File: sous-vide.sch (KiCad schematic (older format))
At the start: 25 parts, among them J2 Conn_01x02, J3 Conn_01x02, J5 Conn_01x02, Q1 2N3904, SW1 SW_Push_Dual, SW2 SW_Push_Dual, U1 node_mcu1.0, U2 RAC01, U3 G5LE, U4 LCD_Backpack, U5 P090S-04F20BR10K

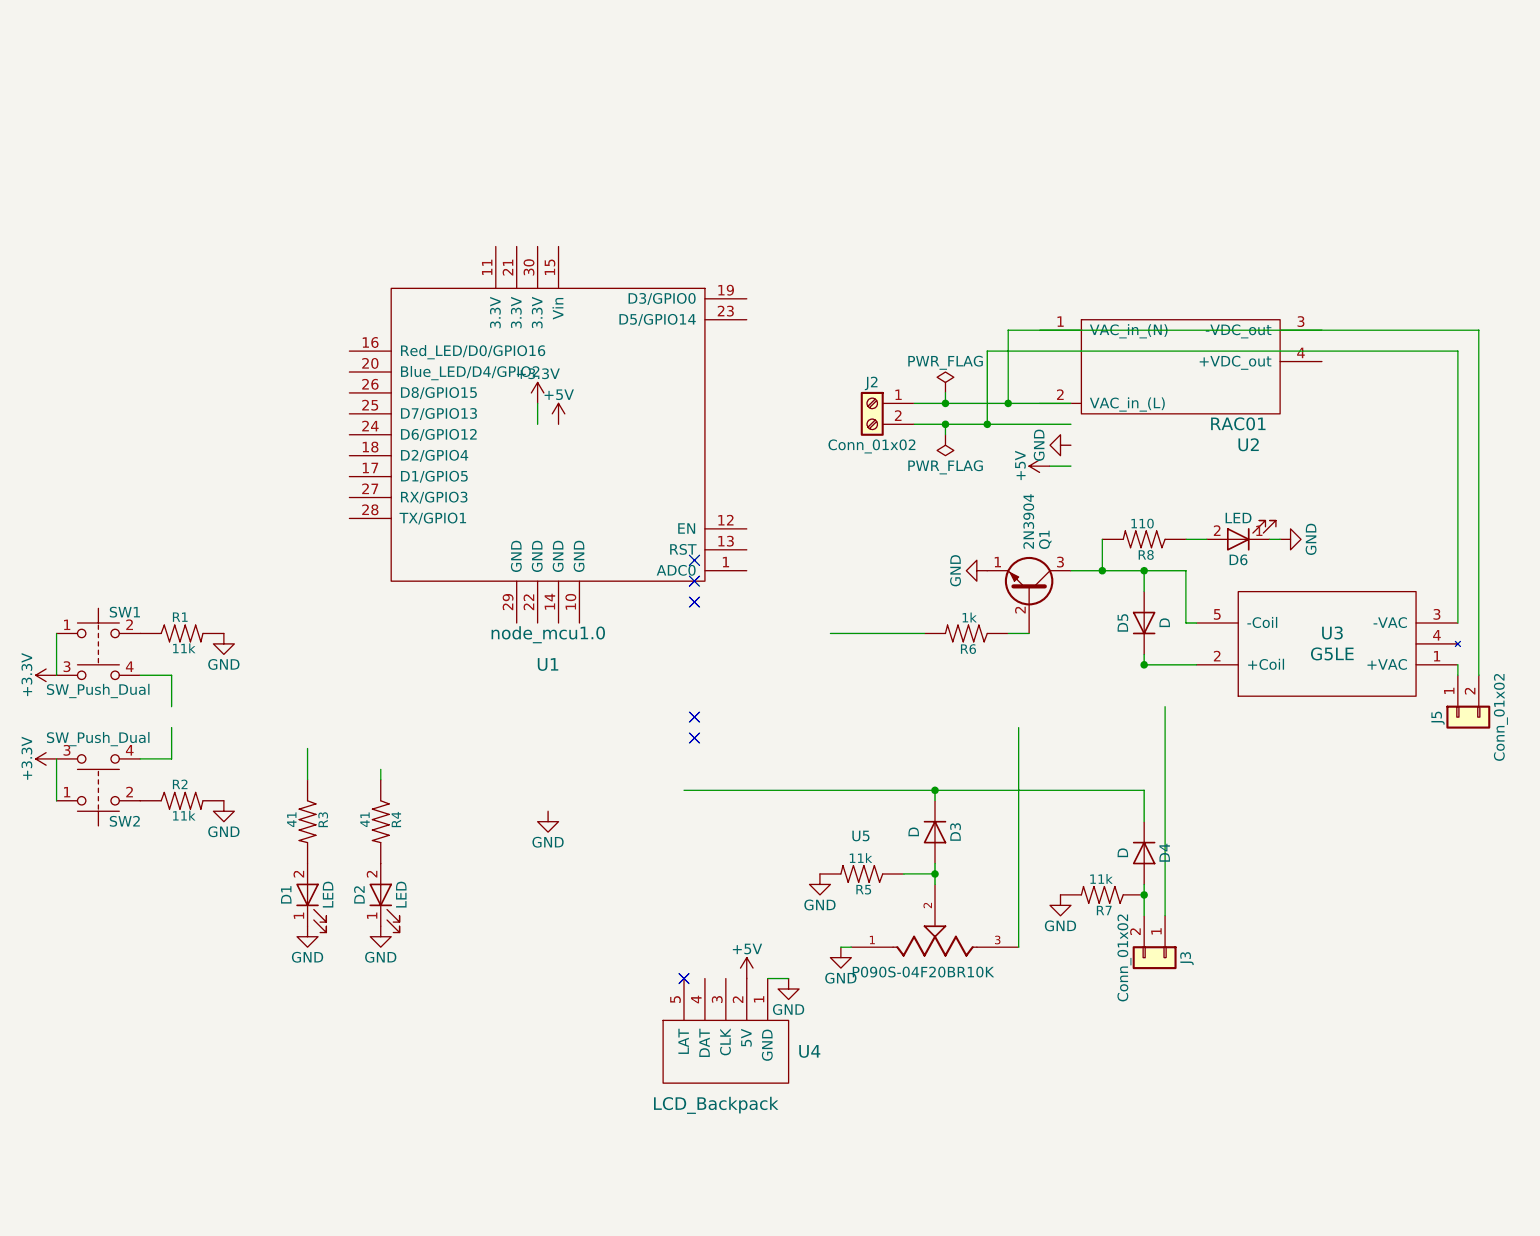
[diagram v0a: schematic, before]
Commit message: redo entire schematic and layout
now complete with danger zone!
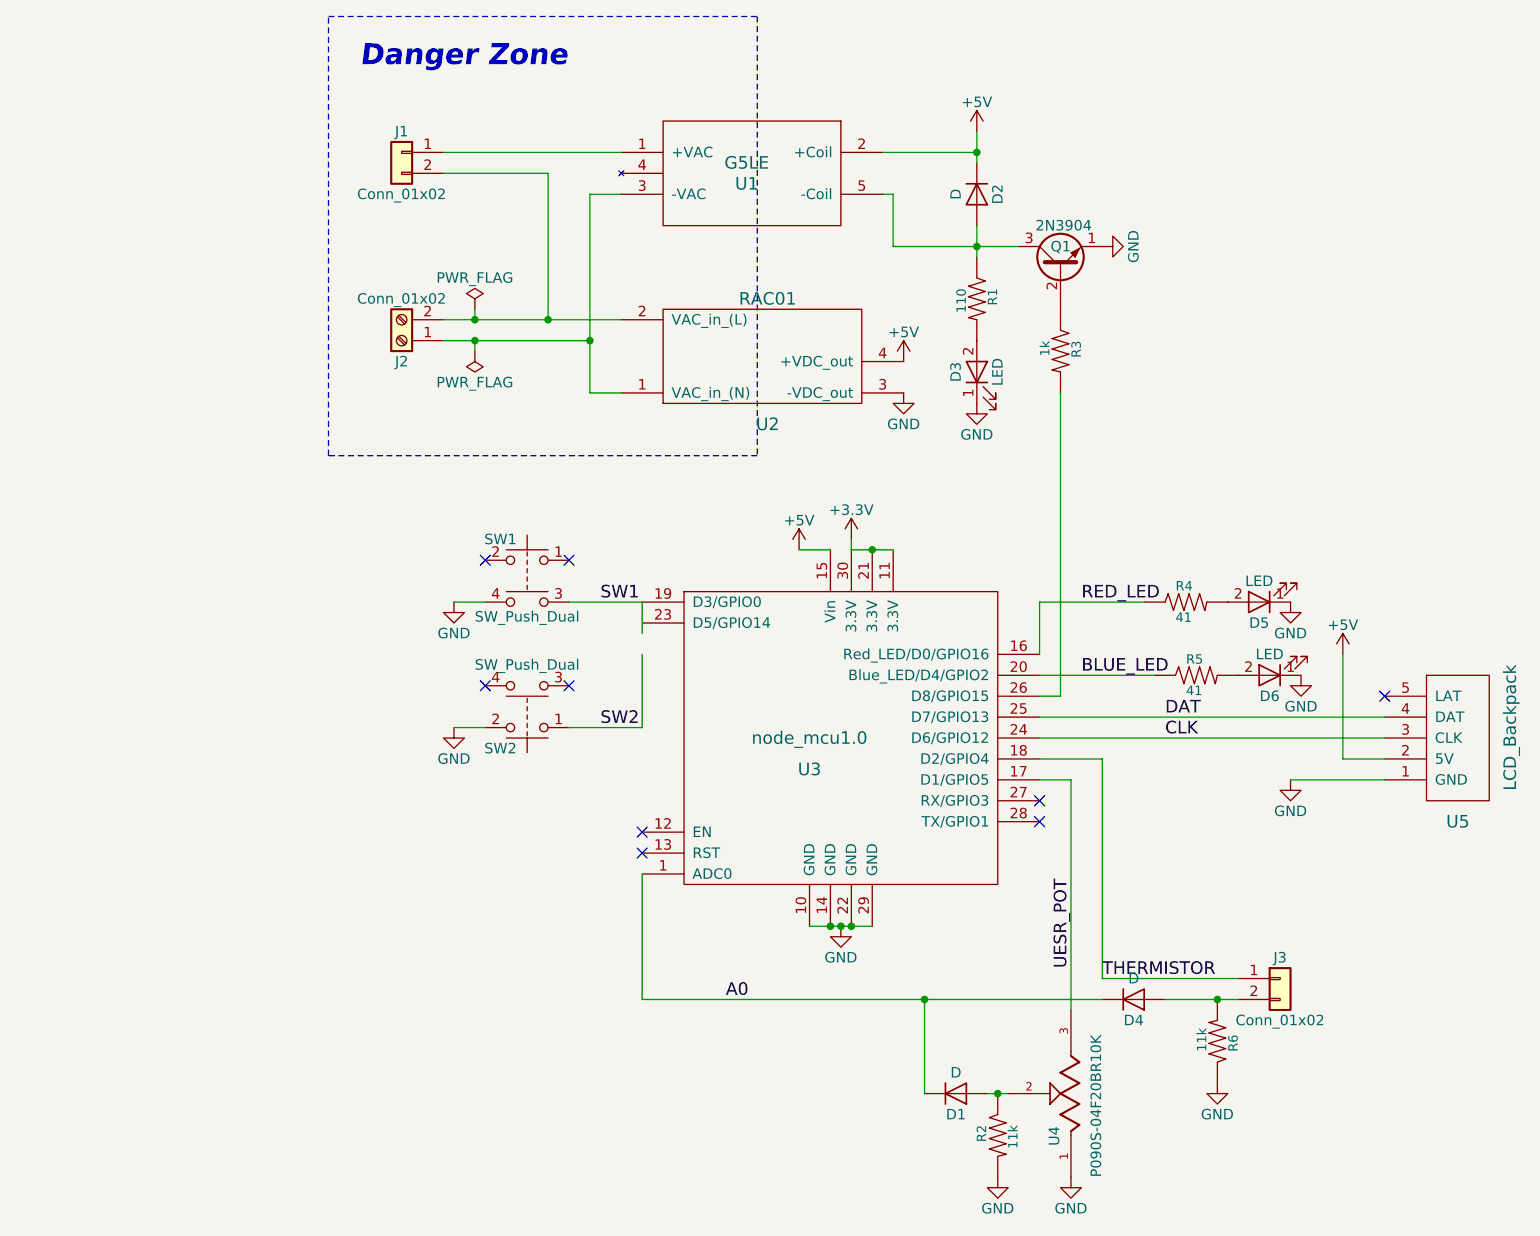
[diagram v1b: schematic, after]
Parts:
- removed R1, R2: 11k, Resistors_THT:R_Axial_DIN0204_L3.6mm_D1.6mm_P7.62mm_Horizontal, symbol RESISTOR0402
- renumbered D3 to D1, D5 to D2, D6 to D3, D2 to D5, D1 to D6, J5 to J1, R8 to R1, R5 to R2, R6 to R3, R3 to R5, R7 to R6, U3 to U1, U1 to U3, U5 to U4, U4 to U5
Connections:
- net labels added: A0, BLUE_LED, CLK, DAT, RED_LED, SW1, SW2, THERMISTOR, UESR_POT
- wire segments 43 -> 60
- no-connect marks 6 -> 9
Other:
- note added: "Danger Zone"
- moved on the sheet: D1, D2, D3, D4, D5, D6, J1, J2, J3, Q1, R1, R2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
